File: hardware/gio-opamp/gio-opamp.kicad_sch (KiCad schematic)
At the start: 46 parts, among them J1 PJ3001F, J2 PJ3001F, J3 PJ3001F, J4 PJ3001F, U1 TL072, U2 MCP3208, U3 DAC8552, U4 XIAO-RP2350-DIP, U5 TL072

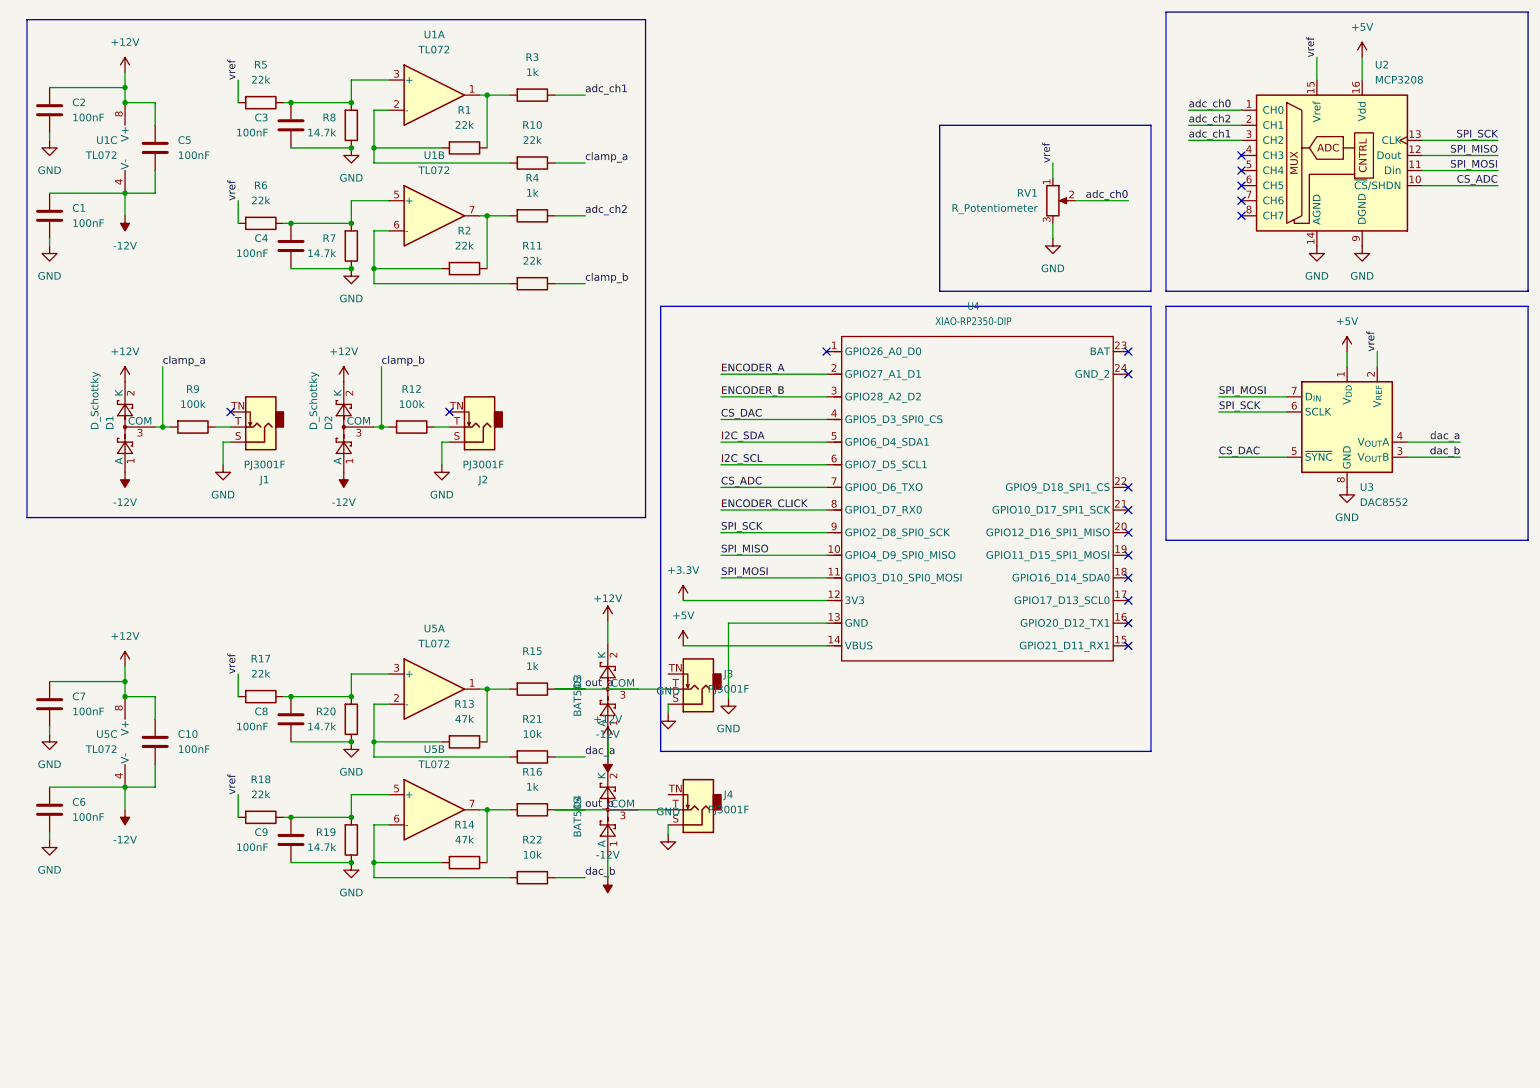
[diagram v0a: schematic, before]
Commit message: routing pcb
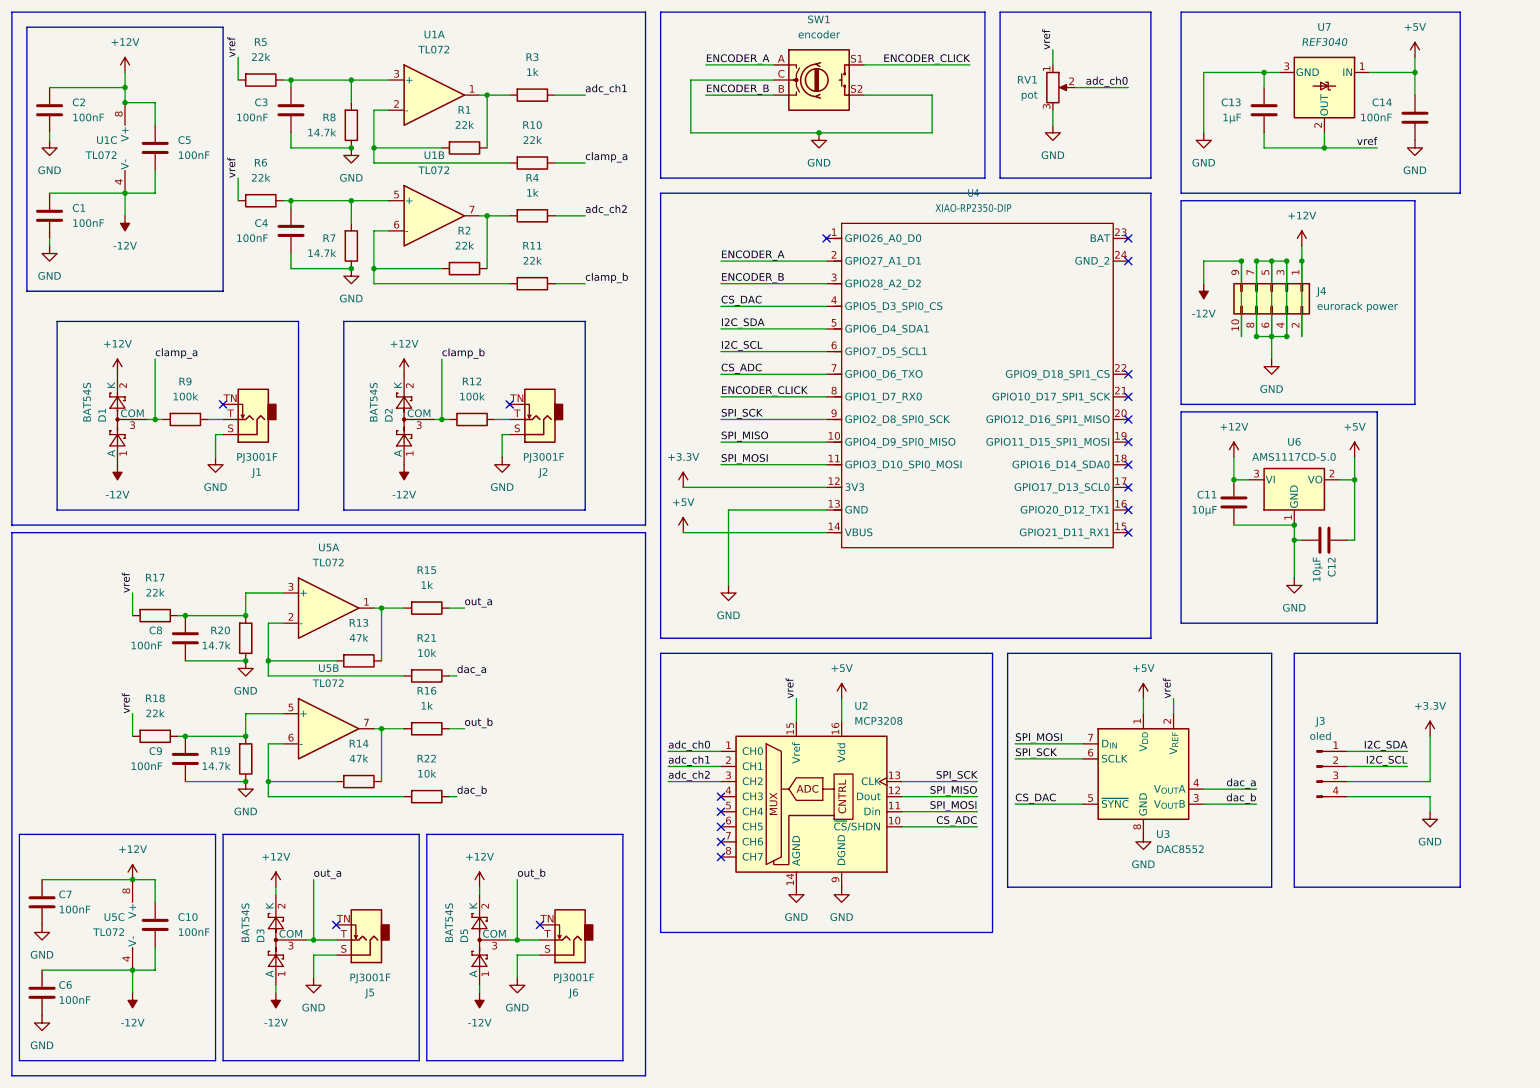
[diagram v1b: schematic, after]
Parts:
- removed D4: BAT54S, symbol Diode:BAT54S
- removed J3, J4: PJ3001F, symbol benjiaomodular:PJ3001F
- added C11, C12: 10µF, Capacitor_SMD:C_0805_2012Metric, symbol Device:C
- added C13: 1µF, Capacitor_SMD:C_0805_2012Metric, symbol Device:C
- added C14: 100nF, Capacitor_SMD:C_0805_2012Metric, symbol Device:C
- added D5: BAT54S, Package_TO_SOT_SMD:SOT-23, symbol Diode:BAT54S
- added J3: oled, Connector_PinHeader_1.27mm:PinHeader_1x04_P1.27mm_Vertical, symbol Connector:Conn_01x04_Pin
- added J4: eurorack power, Connector_PinHeader_2.54mm:PinHeader_1x04_P2.54mm_Vertical, symbol Connector_Generic:Conn_02x05_Odd_Even
- added J5, J6: PJ3001F, Connector_Audio:Jack_3.5mm_QingPu_WQP-PJ398SM_Vertical_CircularHoles, symbol benjiaomodular:PJ3001F
- added SW1: encoder, Rotary_Encoder:RotaryEncoder_Bourns_Vertical_PEC12R-3x17F-Sxxxx, symbol Device:RotaryEncoder_Switch
- added U6: AMS1117CD-5.0, Package_TO_SOT_SMD:TO-252-3_TabPin2, symbol Regulator_Linear:AMS1117CD-5.0
- added U7: REF3040, Package_TO_SOT_SMD:SOT-23, symbol Reference_Voltage:REF3040
- C1, C10, C2, C3, C4, C5, C6, C7, C8, C9: footprint (none) -> Capacitor_SMD:C_0805_2012Metric
- D1, D2: value D_Schottky -> BAT54S
- D3: footprint (none) -> Package_TO_SOT_SMD:SOT-23
- J1, J2: footprint (none) -> Connector_Audio:Jack_3.5mm_QingPu_WQP-PJ398SM_Vertical_CircularHoles
- R1, R10, R11, R12, R13, R14, R15, R16, R17, R18, R19, R2, R20, R21, R22, R3, R4, R5, R6, R7, R8, R9: footprint (none) -> Resistor_SMD:R_0805_2012Metric
- RV1: value R_Potentiometer -> pot; footprint (none) -> benjiaomodular:Potentiometer_RV09
- U1, U5: footprint (none) -> Package_SO:SO-8_3.9x4.9mm_P1.27mm
- U2: footprint (none) -> Package_SO:SOIC-16_3.9x9.9mm_P1.27mm
- U4: footprint Seeed_Studio_XIAO_Series:XIAO-RP2350-DIP -> Seeed Studio XIAO Series Library:XIAO-RP2350-DIP
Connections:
- net +12V: now also C11.1, D5.2 (K), J4.1 (Pin_1), J4.2 (Pin_2), U6.3 (VI); no longer C1.1, C10.2, C5.2, C6.1, D1.1 (A), D2.1 (A), D3.1 (A), U1.4 (V-), U5.4 (V-)
- net +3.3V: now also J3.3 (Pin_3)
- net +5V: now also C12.1, C14.1, U6.2 (VO), U7.1 (IN)
- net ENCODER_A: now also SW1.A
- net ENCODER_B: now also SW1.B
- net ENCODER_CLICK: now also SW1.S1
- net GND: now also C11.2, C12.2, C13.1, C14.2, J3.4 (Pin_4), J4.3 (Pin_3), J4.4 (Pin_4), J4.5 (Pin_5), J4.6 (Pin_6), J4.7 (Pin_7), J4.8 (Pin_8), J5.S, J6.S, SW1.C, SW1.S2, U6.1 (GND), U7.3 (GND)
- net I2C_SCL: now also J3.2 (Pin_2)
- net I2C_SDA: now also J3.1 (Pin_1)
- net adc_ch1: now also U2.2 (CH1); no longer U2.3 (CH2)
- net adc_ch2: now also U2.3 (CH2); no longer U2.2 (CH1)
- net out_a: now also J5.T
- net out_b: now also D5.3 (COM), J6.T
- net vref: now also C13.2, U7.2 (OUT)
- new net -12V: C1.1, C10.2, C5.2, C6.1, D1.1 (A), D2.1 (A), D3.1 (A), D5.1 (A), J4.10 (Pin_10), J4.9 (Pin_9), U1.4 (V-), U5.4 (V-)
- no-connect marks 18 -> 20
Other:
- company: (none) -> funkfinger
- title: (none) -> gio
- moved on the sheet: C10, C3, C4, C6, C7, C8, C9, D1, D2, J1, J2, R12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
